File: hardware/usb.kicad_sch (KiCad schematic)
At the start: 18 parts, among them J3 USB_C_Receptacle, Q2 MBT2222ADW1T1, U10 CP2102N-Axx-xQFN24

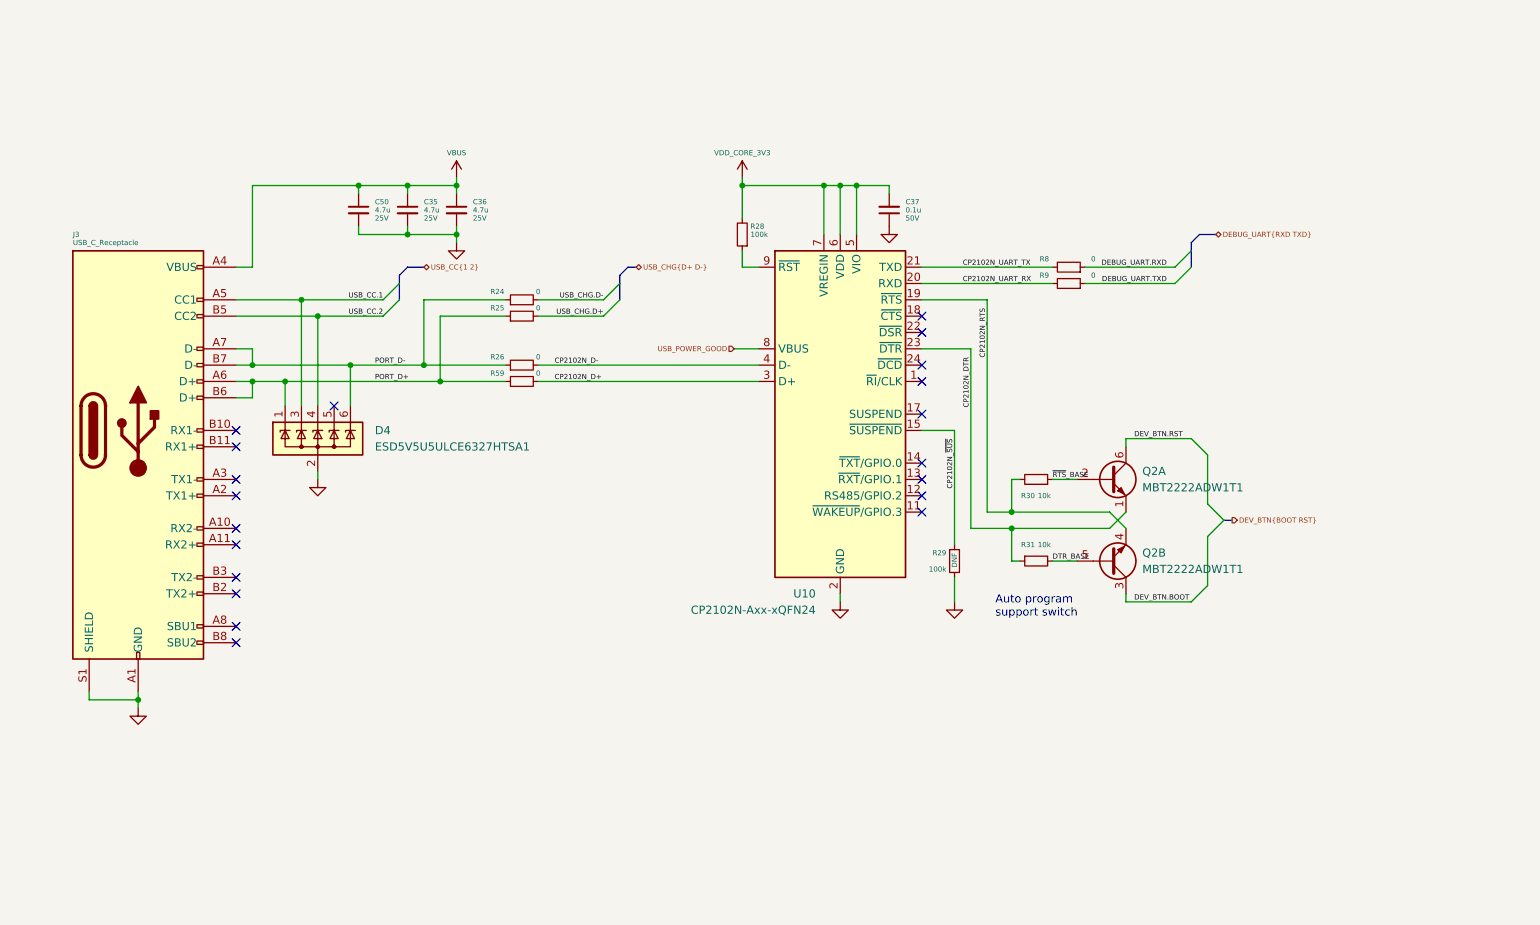
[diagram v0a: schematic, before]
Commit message: Updates
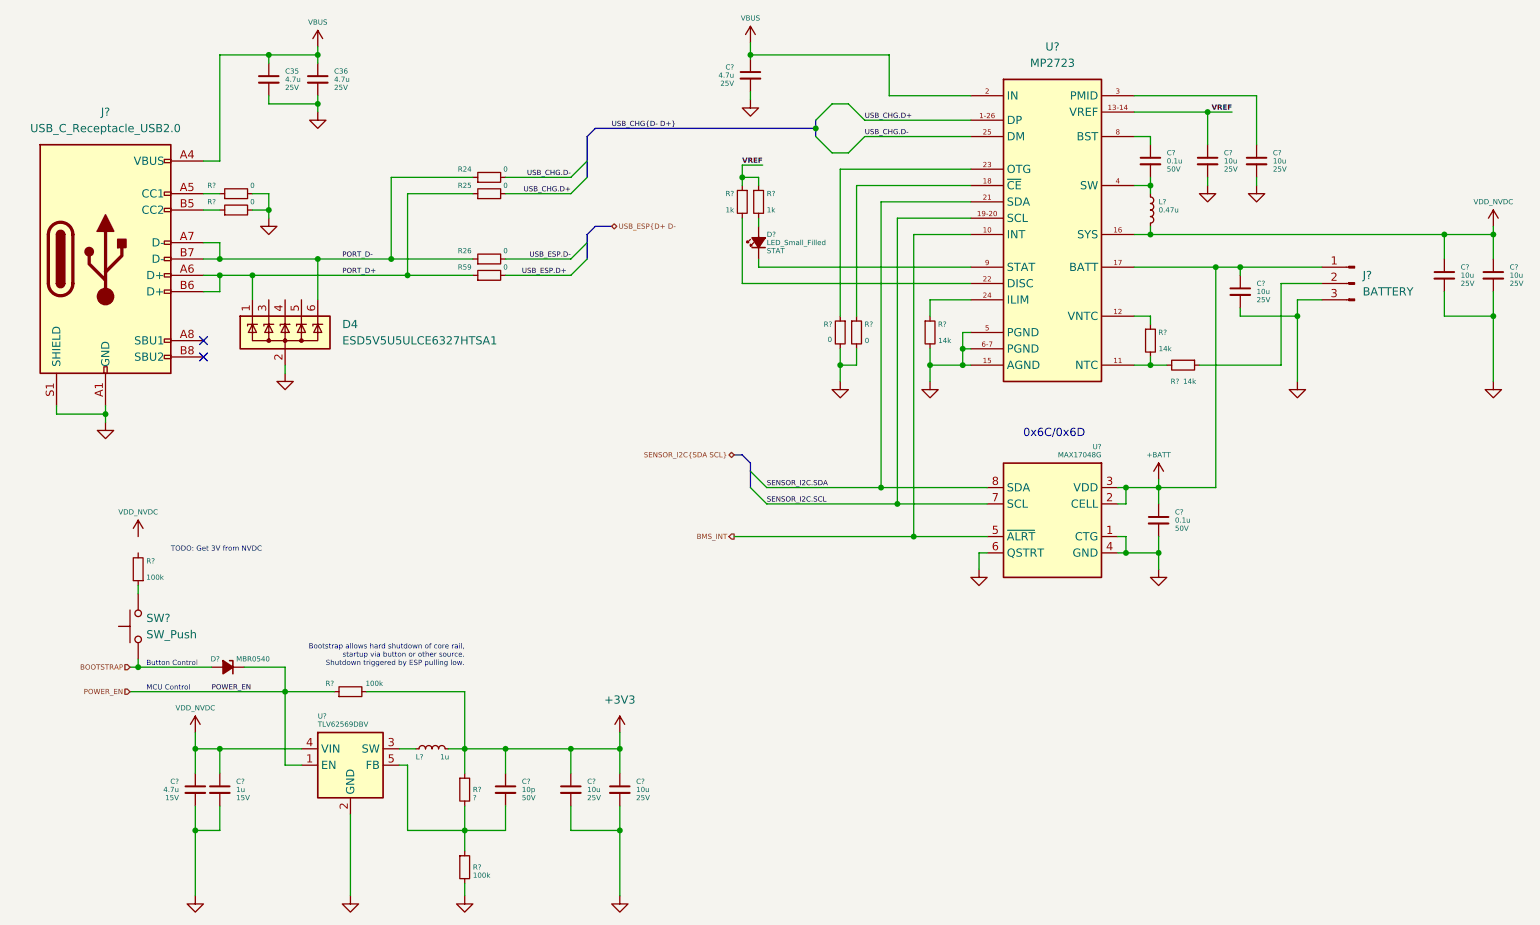
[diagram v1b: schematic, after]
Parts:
- removed C37: 0.1u, Capacitor_SMD:C_0402_1005Metric, symbol Device:C_Small
- removed C50: 4.7u, Capacitor_SMD:C_0603_1608Metric, symbol Device:C_Small
- removed J3: USB_C_Receptacle, bt_Connector_USB:AMPHENOL_124019032112A, symbol Connector:USB_C_Receptacle
- removed Q2: MBT2222ADW1T1, Package_TO_SOT_SMD:SOT-363_SC-70-6, symbol Transistor_BJT:MBT2222ADW1T1
- removed R28, R29: 100k, Resistor_SMD:R_0402_1005Metric, symbol Device:R_Small
- removed R30, R31: 10k, Resistor_SMD:R_0402_1005Metric, symbol Device:R_Small
- removed R8, R9: 0, Resistor_SMD:R_0402_1005Metric, symbol Device:R_Small
- removed U10: CP2102N-Axx-xQFN24, Package_DFN_QFN:QFN-24-1EP_4x4mm_P0.5mm_EP2.6x2.6mm, symbol Interface_USB:CP2102N-Axx-xQFN24
- added C? (x2): 4.7u, Capacitor_SMD:C_0603_1608Metric, symbol Device:C_Small
- added C?: 10p, Capacitor_SMD:C_0402_1005Metric, symbol Device:C_Small
- added C? (x7): 10u, Capacitor_SMD:C_0603_1608Metric, symbol Device:C_Small
- added C? (x2): 0.1u, Capacitor_SMD:C_0402_1005Metric, symbol Device:C_Small
- added C?: 1u, Capacitor_SMD:C_0402_1005Metric, symbol Device:C_Small
- added D?: MBR0540, LED_SMD:LED_0603_1608Metric, symbol Device:D_Zener_Small_Filled
- added D?: LED_Small_Filled, LED_SMD:LED_0402_1005Metric, symbol Device:LED_Small_Filled
- added J?: USB_C_Receptacle_USB2.0, symbol Connector:USB_C_Receptacle_USB2.0
- added J?: BATTERY, symbol Connector:Conn_01x03_Male
- added L?: 1u, Inductor_SMD:L_Wuerth_MAPI-2510, symbol Device:L_Small
- added L?: 0.47u, Inductor_SMD:L_Wuerth_MAPI-2510, symbol Device:L_Small
- added R? (x4): 0, Resistor_SMD:R_0402_1005Metric, symbol Device:R_Small
- added R? (x3): 14k, Resistor_SMD:R_0402_1005Metric, symbol Device:R_Small
- added R? (x3): 100k, Resistor_SMD:R_0402_1005Metric, symbol Device:R_Small
- added R? (x2): 1k, Resistor_SMD:R_0402_1005Metric, symbol Device:R_Small
- added R?: ?, Resistor_SMD:R_0402_1005Metric, symbol Device:R_Small
- added SW?: SW_Push, symbol Switch:SW_Push
- added U?: MP2723, bt_Package_QFN:MP_QFN-26-3.5x3.5_P0.45mm, symbol bt_PMIC_Battery_Charger:MP2723
- added U?: TLV62569DBV, Package_TO_SOT_SMD:SOT-23-5, symbol Regulator_Switching:TLV62569DBV
- added U?: MAX17048G, Package_DFN_QFN:TDFN-8-1EP_2x2mm_P0.5mm_EP0.8x1.2mm, symbol bt_PMIC_Battery_Management:MAX17048G
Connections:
- net GND: now also C?.2, C?.2, C?.2, C?.2, C?.2, C?.2, C?.2, C?.2, C?.2, C?.2, C?.2, J?.3 (Pin_3), J?.A1 (GND), J?.A12 (GND), J?.B1 (GND), J?.B12 (GND), J?.S1 (SHIELD), R?.2, R?.2, R?.2, R?.2, R?.2, R?.2, U?.1 (CTG), U?.15 (AGND), U?.2 (GND), U?.4 (GND), U?.5 (PGND), U?.6 (QSTRT), U?.6-7 (PGND)
- net PORT_D+: now also J?.A6 (D+), J?.B6 (D+)
- net PORT_D-: now also J?.A7 (D-), J?.B7 (D-)
- net USB_CHG.D+: now also U?.1-26 (DP)
- net USB_CHG.D-: now also U?.25 (DM)
- net VBUS: now also C?.1, J?.A4 (VBUS), J?.A9 (VBUS), J?.B4 (VBUS), J?.B9 (VBUS), U?.2 (IN)
- net CP2102N_D+ renamed USB_ESP.D+
- net CP2102N_D- renamed USB_ESP.D-
- net USB_CC.1: no longer names the net of D4.3 (K)
- net USB_CC.2: no longer names the net of D4.4 (K)
- new net: L?.1, U?.3 (SW)
- new net: C?.2, R?.1, R?.2, U?.5 (FB)
- new net: J?.B5 (CC2), R?.1
- new net: R?.1, U?.12 (VNTC)
- new net: R?.2, R?.2, U?.11 (NTC)
- new net: R?.1, U?.24 (ILIM)
- new net: R?.1, U?.23 (OTG)
- new net: J?.A5 (CC1), R?.1
- new net: J?.2 (Pin_2), R?.1
- new net: D?.2 (A), R?.2
- new net: R?.1, U?.18 (~{CE})
- new net: R?.2, U?.22 (DISC)
- new net: C?.1, U?.3 (PMID)
- new net: C?.2, L?.1, U?.4 (SW)
- new net: C?.1, U?.8 (BST)
- new net: D?.1 (K), U?.9 (STAT)
- new net: R?.1, SW?.1
- new net +3V3: C?.1, C?.1, C?.1, L?.2, R?.1, R?.2
- new net +BATT: C?.1, C?.1, J?.1 (Pin_1), U?.17 (BATT), U?.2 (CELL), U?.3 (VDD)
- new net BMS_INT: U?.10 (INT), U?.5 (~{ALRT})
- new net BOOTSTRAP: D?.2 (A), SW?.2
- new net POWER_EN: D?.1 (K), R?.1, U?.1 (EN)
- new net SENSOR_I2C.SCL: U?.19-20 (SCL), U?.7 (SCL)
- new net SENSOR_I2C.SDA: U?.21 (SDA), U?.8 (SDA)
- new net VDD_NVDC: C?.1, C?.1, C?.1, C?.1, L?.2, U?.16 (SYS), U?.4 (VIN)
- new net VREF: C?.1, R?.1, R?.1, U?.13-14 (VREF)
- no-connect marks 20 -> 2
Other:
- note added: "0x6C/0x6D"
- note added: "Bootstrap allows hard shutdown of core rail, startup via button or other source. Shutdown triggered by ESP pulling low."
- note added: "Button Control"
- note added: "MCU Control"
- note added: "TODO: Get 3V from NVDC"
- note removed: "Auto program support switch"
- moved on the sheet: C35, C36, D4, R24, R25, R26, R59
